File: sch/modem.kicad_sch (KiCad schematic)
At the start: 48 parts, among them J10 TestPoint, J11 TestPoint, J12 TestPoint, J13 TestPoint, J14 TestPoint, J18 3V7_in, J4 EMPCB.SMAFSTJ.B.HT, J5 EMPCB.SMAFSTJ.B.HT, J6 TestPoint, J7 TestPoint, J8 TestPoint, J9 TestPoint, P1 SF72S006VBDR2500, U1 RC7620_1105027, U2 NX3008NBKW_115, U3 NX3008NBKW_115, U4 NX3008NBKW_115, U5 NX3008NBKW_115, U6 NX3008NBKW_115, U7 NX3008NBKW_115

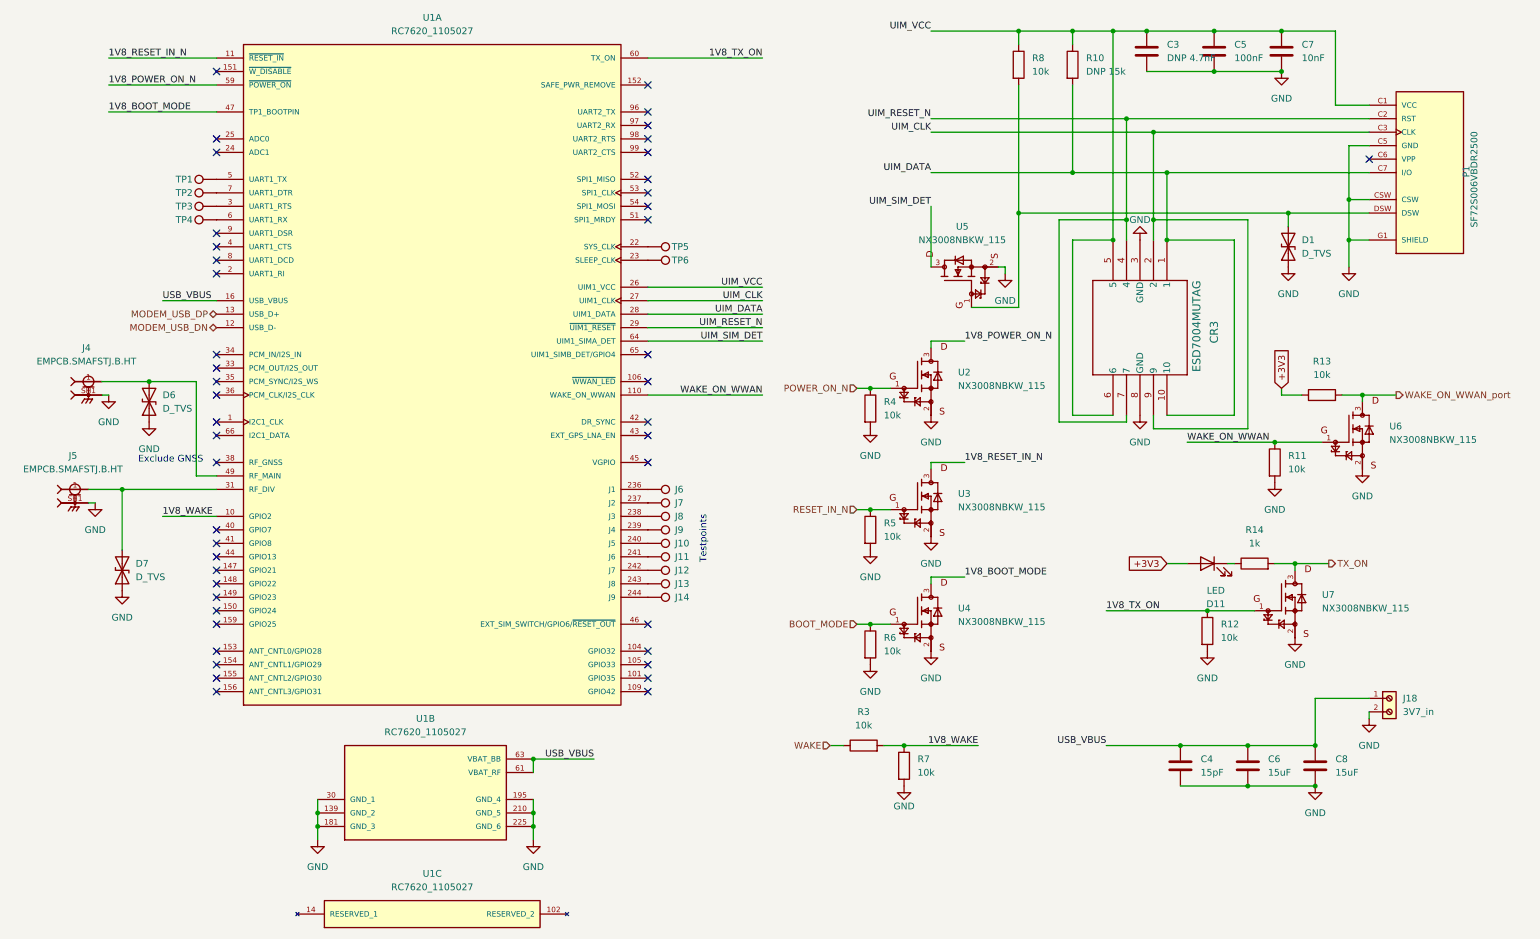
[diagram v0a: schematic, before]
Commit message: pågebynt merging av pwr-supply og modem branches
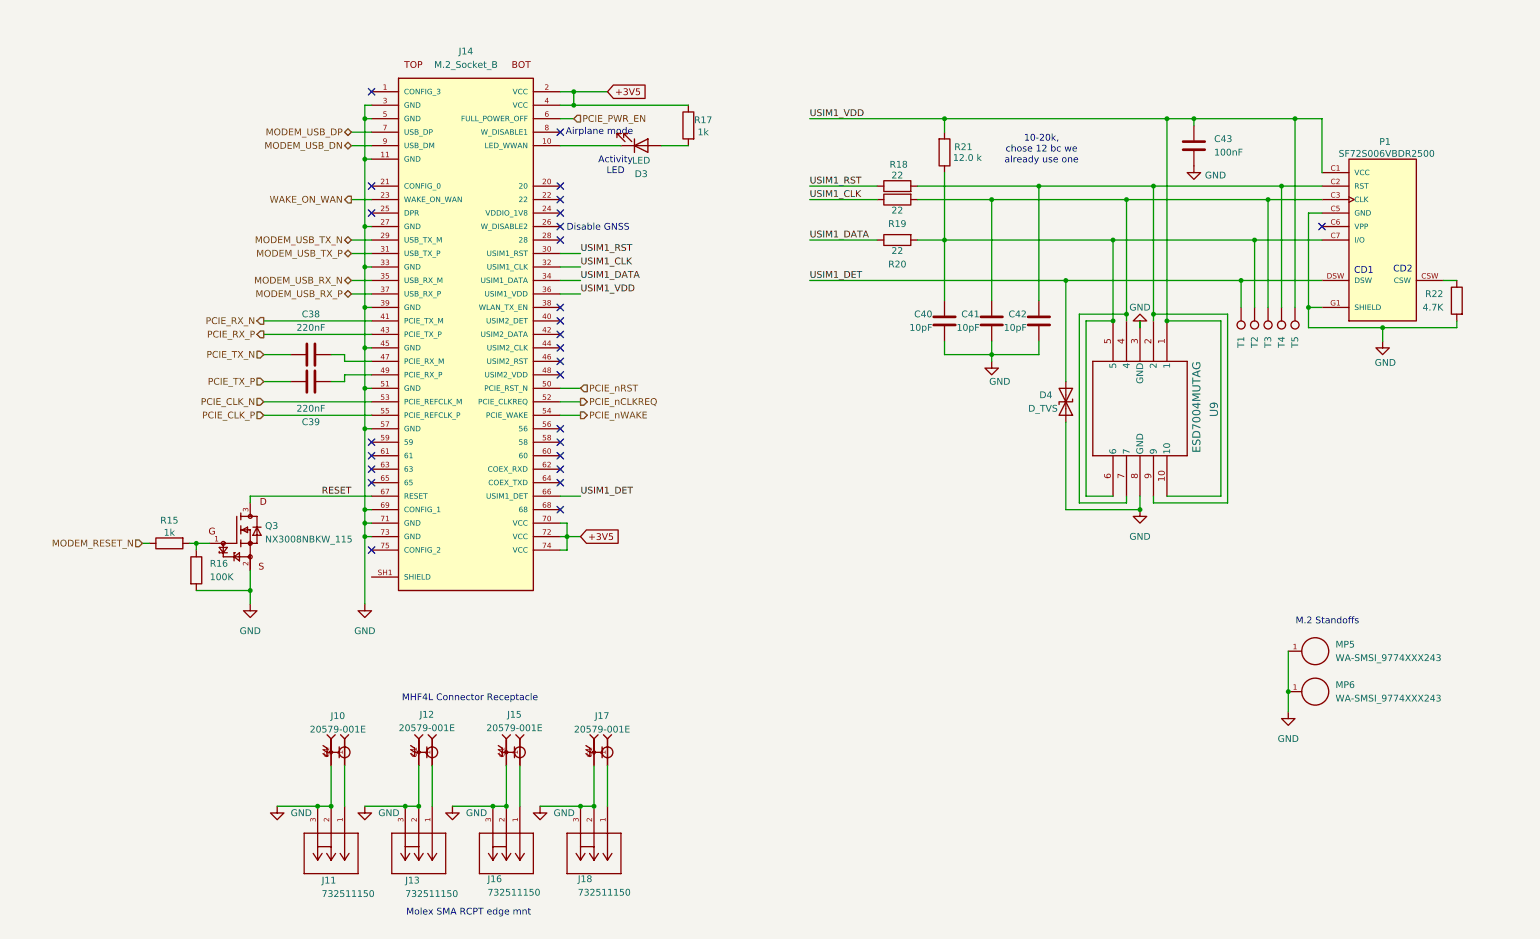
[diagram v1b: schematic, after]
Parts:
- removed C3: DNP 4.7nF, Capacitor_SMD:C_0603_1608Metric, symbol Device:C
- removed C4: 15pF, Capacitor_SMD:C_0603_1608Metric, symbol Device:C
- removed C5: 100nF, Capacitor_SMD:C_0603_1608Metric, symbol Device:C
- removed C6, C8: 15uF, Capacitor_SMD:C_0603_1608Metric, symbol Device:C
- removed C7: 10nF, Capacitor_SMD:C_0603_1608Metric, symbol Device:C
- removed CR3: ESD7004MUTAG, UDFN10_517BB_ONS, symbol ESD7004MUTAG:ESD7004MUTAG
- removed D11: LED, LTST-C190GKT:LEDM1608X80, symbol Device:LED
- removed D6, D7: D_TVS, Diode_SMD:D_0402_1005Metric, symbol Device:D_TVS
- removed J10, J11, J12, J13, J14, J6, J7, J8, J9: TestPoint, TestPoint:TestPoint_Loop_D2.50mm_Drill1.0mm, symbol Connector:TestPoint
- removed J18: 3V7_in, 691137710002:691137710002, symbol 691137710002:691137710002
- removed J4, J5: EMPCB.SMAFSTJ.B.HT, EMPCB.SMAFSTJ.B.HT:TAOGLAS_EMPCB.SMAFSTJ.B.HT, symbol EMPCB.SMAFSTJ.B.HT:EMPCB.SMAFSTJ.B.HT
- removed R10: DNP 15k, Resistor_SMD:R_0603_1608Metric, symbol Device:R
- removed R11, R12, R13, R3, R4, R5, R6, R7, R8: 10k, Resistor_SMD:R_0603_1608Metric, symbol Device:R
- removed R14: 1k, Resistor_SMD:R_0603_1608Metric, symbol Device:R
- removed TP1, TP2, TP3, TP4: T1, TestPoint:TestPoint_Loop_D2.50mm_Drill1.0mm, symbol Connector:TestPoint
- removed TP5, TP6: T1, TestPoint:TestPoint_Pad_D1.5mm, symbol Connector:TestPoint
- removed U1: RC7620_1105027, RC7620_1104625:XCVR_RC7620_1104625, symbol RC7620_1104625:RC7620_1104625
- removed U2, U3, U4, U5, U6, U7: NX3008NBKW_115, NX3008NBKW_115:SOT65P210X110-3N, symbol NX3008NBKW_115:NX3008NBKW_115
- added C38, C39: 220nF, Capacitor_SMD:C_0603_1608Metric, symbol Device:C
- added C40, C41, C42: 10pF, Capacitor_SMD:C_0603_1608Metric, symbol Device:C
- added C43: 100nF, Capacitor_SMD:C_0603_1608Metric, symbol Device:C
- added D3: LED, LTST-C190GKT:LEDM1608X80, symbol Device:LED
- added J10, J12, J15, J17: 20579-001E, 20579-001E:IPEX_20579-001E, symbol 20579-001E:20579-001E
- added J11, J13, J16, J18: 732511150, 732511150:CONN_73251-1150_MOL, symbol 732511150:732511150
- added J14: M.2_Socket_B, 2199119-3:TE_2199119-3, symbol 2199119-3:2199119-3
- added MP5, MP6: WA-SMSI_9774XXX243, WA-SMSI_9774XXX243:WA-SMSI_9774030243, symbol WA-SMSI_9774XXX243:WA-SMSI_9774XXX243
- added Q3: NX3008NBKW_115, NX3008NBKW_115:SOT65P210X110-3N, symbol NX3008NBKW_115:NX3008NBKW_115
- added R15, R17: 1k, Resistor_SMD:R_0603_1608Metric, symbol Device:R
- added R16: 100K, Resistor_SMD:R_0603_1608Metric, symbol Device:R
- added R18, R19, R20: 22, Resistor_SMD:R_0603_1608Metric, symbol Device:R
- added R21: 12.0 k, Resistor_SMD:R_0603_1608Metric, symbol Device:R
- added R22: 4.7K, Resistor_SMD:R_0603_1608Metric, symbol Device:R
- added T1, T2, T3, T4, T5: TestPoint, TestPoint:TestPoint_Loop_D2.60mm_Drill1.6mm_Beaded, symbol Connector:TestPoint
- added U9: ESD7004MUTAG, ESD7004MUTAG:UDFN10_517BB_ONS, symbol ESD7004MUTAG:ESD7004MUTAG
- renumbered D1 to D4
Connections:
- net GND: now also C40.2, C41.2, C42.2, C43.2, J10.G1, J10.G2, J10.G3, J11.2, J11.3, J12.G1, J12.G2, J12.G3, J13.2, J13.3, J14.11 (GND), J14.27 (GND), J14.3 (GND), J14.33 (GND), J14.39 (GND), J14.45 (GND), J14.5 (GND), J14.51 (GND), J14.57 (GND), J14.69 (CONFIG_1), J14.71 (GND), J14.73 (GND), J15.G1, J15.G2, J15.G3, J16.2, J16.3, J17.G1, J17.G2, J17.G3, J18.2, J18.3, MP5.1, MP6.1, Q3.2, R16.2, R22.2, U9.3 (GND), U9.8 (GND); no longer P1.CSW
- net MODEM_USB_DN: now also J14.9 (USB_DM)
- net MODEM_USB_DP: now also J14.7 (USB_DP)
- net USIM1_DET: now reaches D4.2 (A2), P1.DSW
- net USIM1_DET: now also J14.66 (USIM1_DET), T1.1
- net UIM_CLK: no longer names the net of P1.C3 (CLK)
- net UIM_CLK: now also C41.1, R19.2, T3.1, U9.4, U9.7
- net UIM_DATA: no longer names the net of P1.C7 (I/O)
- net UIM_DATA: now also C40.1, R20.2, R21.1, T2.1, U9.5, U9.6
- net UIM_RESET_N: no longer names the net of P1.C2 (RST)
- net UIM_RESET_N: now also C42.1, R18.2, T4.1, U9.2, U9.9
- net UIM_VCC renamed USIM1_VDD
- net USIM1_VDD: now also C43.1, J14.36 (USIM1_VDD), R21.2, T5.1, U9.1, U9.10
- new net: P1.CSW, R22.1
- new net: J10.1, J11.1
- new net: J15.1, J16.1
- new net: J12.1, J13.1
- new net: C38.2, J14.47 (PCIE_RX_M)
- new net: Q3.1, R15.2, R16.1
- new net: C39.2, J14.49 (PCIE_RX_P)
- new net: D3.1, J14.10 (LED_WWAN)
- new net: D3.2, R17.2
- new net: J17.1, J18.1
- new net: J14.SH1 (SHIELD), J14.SH2 (SHIELD)
- new net +3V5: J14.2 (VCC), J14.4 (VCC), J14.70 (VCC), J14.72 (VCC), J14.74 (VCC), R17.1
- new net MODEM_RESET_N: R15.1
- new net MODEM_USB_RX_N: J14.35 (USB_RX_M)
- new net MODEM_USB_RX_P: J14.37 (USB_RX_P)
- new net MODEM_USB_TX_N: J14.29 (USB_TX_M)
- new net MODEM_USB_TX_P: J14.31 (USB_TX_P)
- new net PCIE_CLK_N: J14.53 (PCIE_REFCLK_M)
- new net PCIE_CLK_P: J14.55 (PCIE_REFCLK_P)
- new net PCIE_PWR_EN: J14.6 (FULL_POWER_OFF)
- new net PCIE_RX_N: J14.41 (PCIE_TX_M)
- new net PCIE_RX_P: J14.43 (PCIE_TX_P)
- new net PCIE_TX_N: C38.1
- new net PCIE_TX_P: C39.1
- new net PCIE_nCLKREQ: J14.52 (PCIE_CLKREQ)
- new net PCIE_nRST: J14.50 (PCIE_RST_N)
- new net PCIE_nWAKE: J14.54 (PCIE_WAKE)
- new net RESET: J14.67 (RESET), Q3.3
- new net USIM1_CLK: J14.32 (USIM1_CLK), R19.1
- new net USIM1_DATA: J14.34 (USIM1_DATA), R20.1
- new net USIM1_RST: J14.30 (USIM1_RST), R18.1
- new net WAKE_ON_WAN: J14.23 (WAKE_ON_WAN)
- no-connect marks 46 -> 27
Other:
- note added: "10-20k, chose 12 bc we already use one"
- note added: "Activity LED"
- note added: "Airplane mode"
- note added: "CD1"
- note added: "CD2"
- note added: "Disable GNSS"
- note added: "M.2 Standoffs"
- note added: "MHF4L Connector Receptacle"
- note added: "Molex SMA RCPT edge mnt"
- note removed: "Exclude GNSS"
- note removed: "Testpoints"
- moved on the sheet: D4, P1
